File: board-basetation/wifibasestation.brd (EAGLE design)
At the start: 49.8 x 22 mm, 33 parts, among them IC1 1117EMP, IC2 STM32F072, IC3 HTU21D, J1 SWD_SHROUD_SMD, X1 ESP-03, X2 SMA-142-0711-821/826

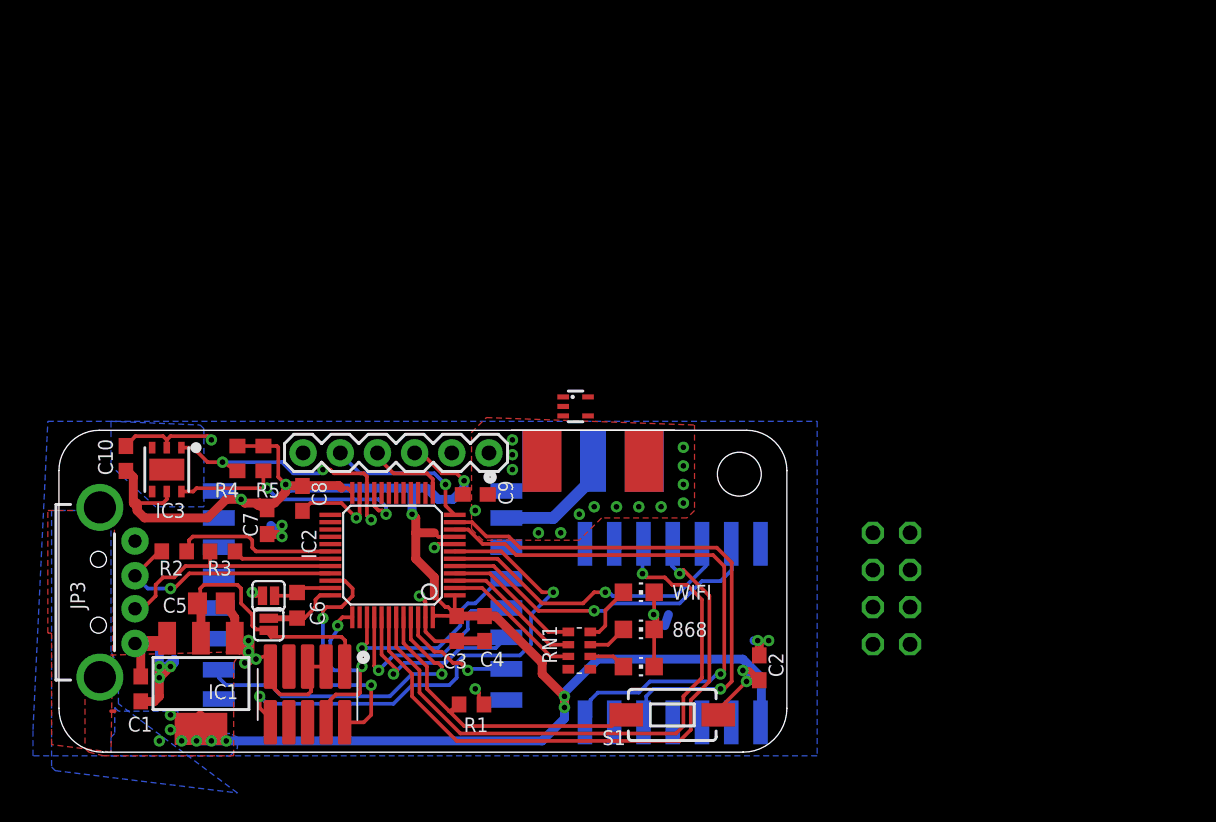
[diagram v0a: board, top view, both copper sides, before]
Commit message: almost done
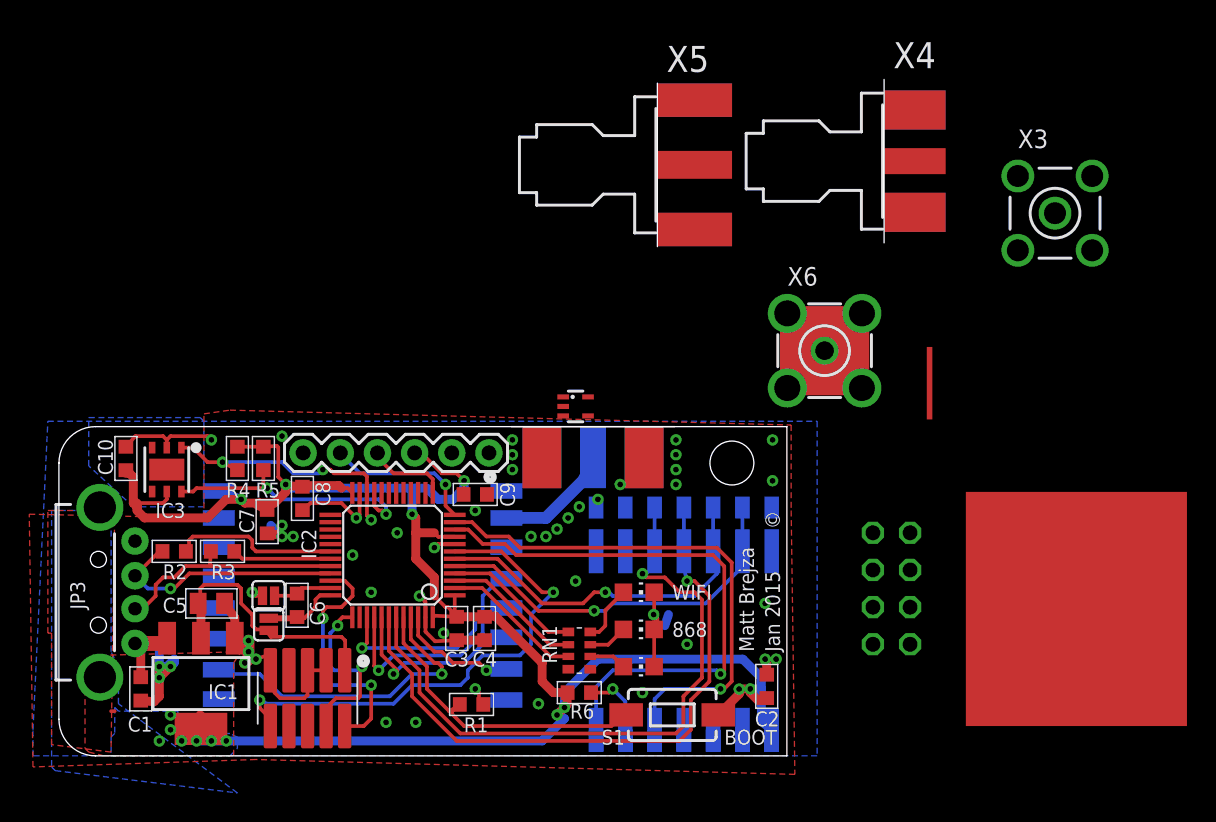
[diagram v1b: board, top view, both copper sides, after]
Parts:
- added R6: 1k, passives-7351:R0603-N
- added U$3: ESP-07, Mine:ESP-07
- added X3: LTI-SASF54GT, con-coax:LTI-SASF54GT
- added X4: SMA-142-0711-821/826, con-coax:J502-ND-142-0711-821/826
- added X5: SMA-142-0711-871/876, con-coax:J502-ND-142-0711-871/876
- added X6: BU-SMA-V, con-coax:BU-SMA-V
- C1, C10, C2, C3, C4, C7, C8, C9: device rcl:C0603 -> passives-7351:C0603-N
- C5: device rcl:C0805 -> passives-7351:C0805-N
- C6: device rcl:C0603K -> passives-7351:C0603-N
- R1, R2, R3, R4, R5: device rcl:R0603 -> passives-7351:R0603-N
- moved C2 1.37 mm to (48.6, 5.00)
- moved X1 0.92 mm to (35.6, 2.03)
- moved X2 0.25 mm to (36.8, 22.8)
- moved J1 0.25 mm to (17.2, 4.19)
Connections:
- new net N$1: R6.2, U$3.6, X1.6
- new net N$3: U$3.2, X1.2
- new net N$4: U$3.4, X1.4
- new net N$7: U$3.3, X1.3
- net +3V3: now also R6.1, U$3.1
- net CH_PD: now also U$3.13
- net GND: now also U$3.8
- net GPIO0: now also U$3.7
- net GPIO15: now also U$3.5
- net USART1_RX: now also U$3.10
- net USART1_TX: now also U$3.11
- net W_RST: now also U$3.12
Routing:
- net N$1: track 0.00 -> 5.50 mm, vias 0 -> 1
- net W_RST: track 21.3 -> 24.9 mm
- net +3V3: track 148.3 -> 151.6 mm
- net CH_PD: track 23.2 -> 26.2 mm
- net USART1_RX: track 41.2 -> 44.2 mm
- net USART1_TX: track 41.5 -> 43.6 mm
- net GPIO0: track 38.2 -> 40.0 mm
- net N$7: track 0.00 -> 0.76 mm
- net N$4: track 0.00 -> 0.76 mm
- net N$3: track 0.00 -> 0.76 mm
- net GND: track 58.6 -> 58.4 mm, vias 33 -> 48
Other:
- board size 49.8 x 22 mm -> 49.8 x 22.5 mm
- board text added: "Add tape to insulate vias"
- board text added: "BOOT"
- board text added: "Jan 2015"
- board text added: "Matt Brejza"
- board text added: "©"
